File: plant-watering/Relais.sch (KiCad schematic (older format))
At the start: 6 parts, among them K1 SRD-05VDC-SL-C, K2 SRD-05VDC-SL-C, K3 SRD-05VDC-SL-C

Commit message: started pcb design
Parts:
- K1, K2, K3: symbol SRD-05VDC-SL-C:SRD-05VDC-SL-C -> plant-watering-rescue:SRD-05VDC-SL-C-SRD-05VDC-SL-C
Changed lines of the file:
@@
 Connection ~ 7250 2750
 $Comp
-L SRD-05VDC-SL-C:SRD-05VDC-SL-C K1
+L plant-watering-rescue:SRD-05VDC-SL-C-SRD-05VDC-SL-C K1
 U 1 1 600B0E95
 P 4250 3400
+AR Path="/600B0E95" Ref="K1"  Part="1"
+AR Path="/600A014F/600B0E95" Ref="K1"  Part="1"
 F 0 "K1" H 4250 3767 50  0000 C CNN
 F 1 "SRD-05VDC-SL-C" H 4250 3676 50  0000 C CNN
@@
 	3750 2750 4650 2750
 $Comp
-L SRD-05VDC-SL-C:SRD-05VDC-SL-C K2
+L plant-watering-rescue:SRD-05VDC-SL-C-SRD-05VDC-SL-C K2
 U 1 1 600B249A
 P 6000 3400
+AR Path="/600B249A" Ref="K2"  Part="1"
+AR Path="/600A014F/600B249A" Ref="K2"  Part="1"
 F 0 "K2" H 6000 3767 50  0000 C CNN
 F 1 "SRD-05VDC-SL-C" H 6000 3676 50  0000 C CNN
@@
 $EndComp
 $Comp
-L SRD-05VDC-SL-C:SRD-05VDC-SL-C K3
+L plant-watering-rescue:SRD-05VDC-SL-C-SRD-05VDC-SL-C K3
 U 1 1 600B35A7
 P 7800 3400
+AR Path="/600B35A7" Ref="K3"  Part="1"
+AR Path="/600A014F/600B35A7" Ref="K3"  Part="1"
 F 0 "K3" H 7800 3767 50  0000 C CNN
 F 1 "SRD-05VDC-SL-C" H 7800 3676 50  0000 C CNN

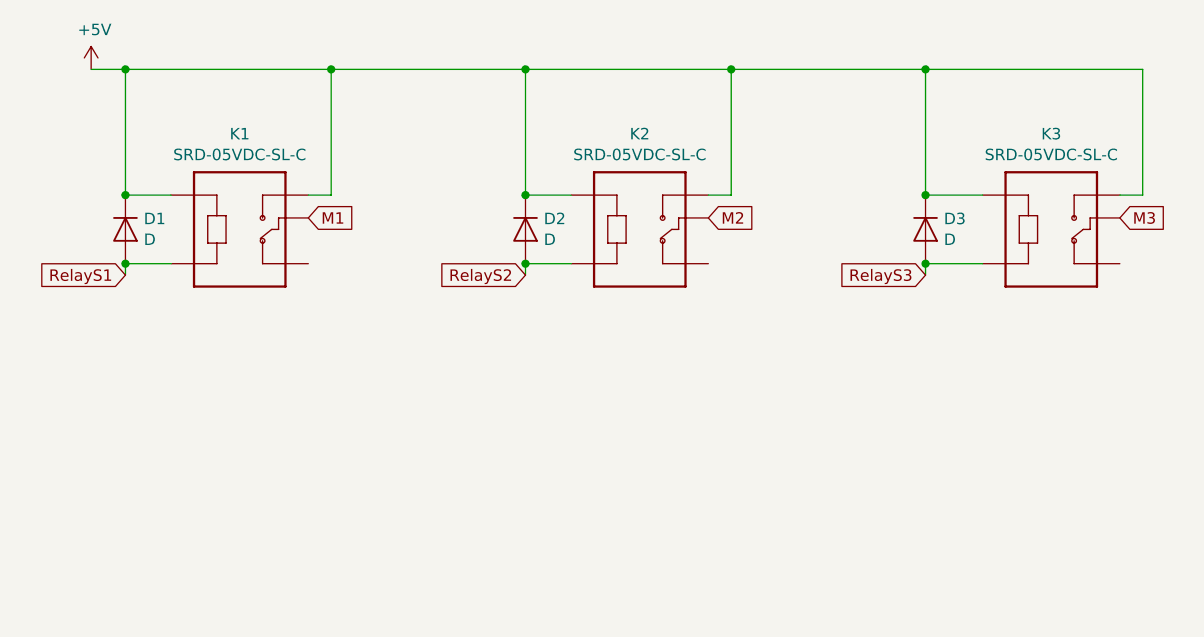
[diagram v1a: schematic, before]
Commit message: added several parts#
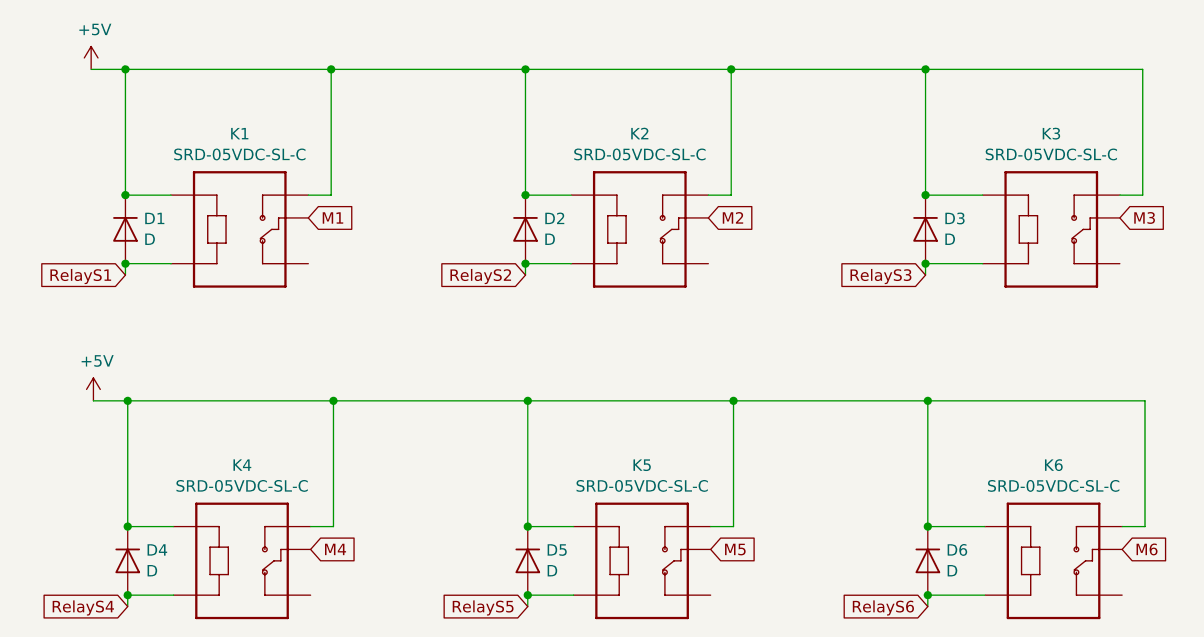
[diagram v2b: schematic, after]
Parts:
- added D4, D5, D6: D, Diodes_ThroughHole:D_DO-41_SOD81_P7.62mm_Horizontal, symbol Device:D
- added K4, K5, K6: SRD-05VDC-SL-C, SRD-05VDC-SL-C:RELAY_SRD-05VDC-SL-C, symbol plant-watering-rescue:SRD-05VDC-SL-C-SRD-05VDC-SL-C
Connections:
- net +5V: now also D4.1 (K), D5.1 (K), D6.1 (K), K4.A1, K4.NO, K5.A1, K5.NO, K6.A1, K6.NO
- new net M4: K4.COM
- new net M5: K5.COM
- new net M6: K6.COM
- new net RelayS4: D4.2 (A), K4.A2
- new net RelayS5: D5.2 (A), K5.A2
- new net RelayS6: D6.2 (A), K6.A2
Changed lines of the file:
@@
 $Descr A4 11693 8268
 encoding utf-8
-Sheet 5 6
+Sheet 5 7
 Title ""
 Date ""
@@
 	5700 3300 5500 3300
 Connection ~ 5500 3300
+$Comp
+L power:+5V #PWR0111
+U 1 1 6011430E
+P 3610 4200
+F 0 "#PWR0111" H 3610 4050 50  0001 C CNN
+F 1 "+5V" H 3625 4373 50  0000 C CNN
+F 2 "" H 3610 4200 50  0001 C CNN
+F 3 "" H 3610 4200 50  0001 C CNN
+	1    3610 4200
+	1    0    0    -1
+$EndComp
+Text GLabel 4560 4850 2    50   Input ~ 0
+M4
+Text GLabel 6310 4850 2    50   Input ~ 0
+M5
+Text GLabel 8110 4850 2    50   Input ~ 0
+M6
+Text GLabel 3760 5100 0    50   Input ~ 0
+RelayS4
+Text GLabel 5510 5100 0    50   Input ~ 0
+RelayS5
+Text GLabel 7260 5100 0    50   Input ~ 0
+RelayS6
+$Comp
+L Device:D D4
+U 1 1 6011431A
+P 3760 4900
+F 0 "D4" V 3714 4980 50  0000 L CNN
+F 1 "D" V 3805 4980 50  0000 L CNN
+F 2 "Diodes_ThroughHole:D_DO-41_SOD81_P7.62mm_Horizontal" H 3760 4900 50  0001 C CNN
+F 3 "~" H 3760 4900 50  0001 C CNN
+	1    3760 4900
+	0    1    1    0
+$EndComp
+$Comp
+L Device:D D5
+U 1 1 60114320
+P 5510 4900
+F 0 "D5" V 5464 4980 50  0000 L CNN
+F 1 "D" V 5555 4980 50  0000 L CNN
+F 2 "Diodes_ThroughHole:D_DO-41_SOD81_P7.62mm_Horizontal" H 5510 4900 50  0001 C CNN
+F 3 "~" H 5510 4900 50  0001 C CNN
+	1    5510 4900
+	0    1    1    0
+$EndComp
+$Comp
+L Device:D D6
+U 1 1 60114326
+P 7260 4900
+F 0 "D6" V 7214 4980 50  0000 L CNN
+F 1 "D" V 7305 4980 50  0000 L CNN
+F 2 "Diodes_ThroughHole:D_DO-41_SOD81_P7.62mm_Horizontal" H 7260 4900 50  0001 C CNN
+F 3 "~" H 7260 4900 50  0001 C CNN
+	1    7260 4900
+	0    1    1    0
+$EndComp
+Wire Wire Line
+	3760 5050 3760 5100
+Wire Wire Line
+	5510 5050 5510 5100
+Wire Wire Line
+	7260 5050 7260 5100
+Connection ~ 3760 4200
+Wire Wire Line
+	3760 4200 3610 4200
+Connection ~ 5510 4200
+Connection ~ 7260 4200
+$Comp
+L plant-watering-rescue:SRD-05VDC-SL-C-SRD-05VDC-SL-C K?
+U 1 1 60114335
+P 4260 4850
+AR Path="/60114335" Ref="K?"  Part="1"
+AR Path="/600A014F/60114335" Ref="K4"  Part="1"
+F 0 "K4" H 4260 5217 50  0000 C CNN
+F 1 "SRD-05VDC-SL-C" H 4260 5126 50  0000 C CNN
+F 2 "SRD-05VDC-SL-C:RELAY_SRD-05VDC-SL-C" H 4260 4850 50  0001 L BNN
+F 3 "" H 4260 4850 50  0001 L BNN
+F 4 "IPC-7251" H 4260 4850 50  0001 L BNN "STANDARD"
+F 5 "SONGLE RELAY" H 4260 4850 50  0001 L BNN "MANUFACTURER"
+	1    4260 4850
+	1    0    0    -1
+$EndComp
+Wire Wire Line
+	3760 4200 3760 4750
+Wire Wire Line
+	3760 4200 4660 4200
+$Comp
+L plant-watering-rescue:SRD-05VDC-SL-C-SRD-05VDC-SL-C K?
+U 1 1 6011433F
+P 6010 4850
+AR Path="/6011433F" Ref="K?"  Part="1"
+AR Path="/600A014F/6011433F" Ref="K5"  Part="1"
+F 0 "K5" H 6010 5217 50  0000 C CNN
+F 1 "SRD-05VDC-SL-C" H 6010 5126 50  0000 C CNN
+F 2 "SRD-05VDC-SL-C:RELAY_SRD-05VDC-SL-C" H 6010 4850 50  0001 L BNN
+F 3 "" H 6010 4850 50  0001 L BNN
+F 4 "IPC-7251" H 6010 4850 50  0001 L BNN "STANDARD"
+F 5 "SONGLE RELAY" H 6010 4850 50  0001 L BNN "MANUFACTURER"
+	1    6010 4850
+	1    0    0    -1
+$EndComp
+$Comp
+L plant-watering-rescue:SRD-05VDC-SL-C-SRD-05VDC-SL-C K?
+U 1 1 60114347
+P 7810 4850
+AR Path="/60114347" Ref="K?"  Part="1"
+AR Path="/600A014F/60114347" Ref="K6"  Part="1"
+F 0 "K6" H 7810 5217 50  0000 C CNN
+F 1 "SRD-05VDC-SL-C" H 7810 5126 50  0000 C CNN
+F 2 "SRD-05VDC-SL-C:RELAY_SRD-05VDC-SL-C" H 7810 4850 50  0001 L BNN
+F 3 "" H 7810 4850 50  0001 L BNN
+F 4 "IPC-7251" H 7810 4850 50  0001 L BNN "STANDARD"
+F 5 "SONGLE RELAY" H 7810 4850 50  0001 L BNN "MANUFACTURER"
+	1    7810 4850
+	1    0    0    -1
+$EndComp
+Wire Wire Line
+	7260 4200 7260 4750
+Wire Wire Line
+	5510 4200 6410 4200
+Wire Wire Line
+	5510 4200 5510 4750
+Wire Wire Line
+	3960 4750 3760 4750
+Connection ~ 3760 4750
+Wire Wire Line
+	3960 5050 3760 5050
+Connection ~ 3760 5050
+Wire Wire Line
+	4560 4750 4660 4750
+Wire Wire Line
+	4660 4750 4660 4200
+Connection ~ 4660 4200
+Wire Wire Line
+	4660 4200 5510 4200
+Wire Wire Line
+	6310 4750 6410 4750
+Wire Wire Line
+	6410 4750 6410 4200
+Connection ~ 6410 4200
+Wire Wire Line
+	6410 4200 7260 4200
+Wire Wire Line
+	7510 4750 7260 4750
+Connection ~ 7260 4750
+Wire Wire Line
+	7510 5050 7260 5050
+Connection ~ 7260 5050
+Wire Wire Line
+	8110 4750 8210 4750
+Wire Wire Line
+	8210 4750 8210 4200
+Wire Wire Line
+	8210 4200 7260 4200
+Wire Wire Line
+	5710 5050 5510 5050
+Connection ~ 5510 5050
+Wire Wire Line
+	5710 4750 5510 4750
+Connection ~ 5510 4750
 $EndSCHEMATC
